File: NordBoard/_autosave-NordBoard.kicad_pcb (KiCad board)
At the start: 2 copper layers, 18 parts, among them SW1 SW_Push, SW10 SW_Push, SW11 SW_Push, SW12 SW_Push, SW13 SW_Push, SW14 SW_Push, SW17 SW_Push, SW18 SW_Push, SW19 SW_Push, SW20 SW_Push, SW21 SW_Push, SW3 SW_Push, SW4 SW_Push, SW5 SW_Push, SW6 SW_Push, SW7 SW_Push, SW8 SW_Push, U1 MOUDLE-SEEEDUINO-XIAO

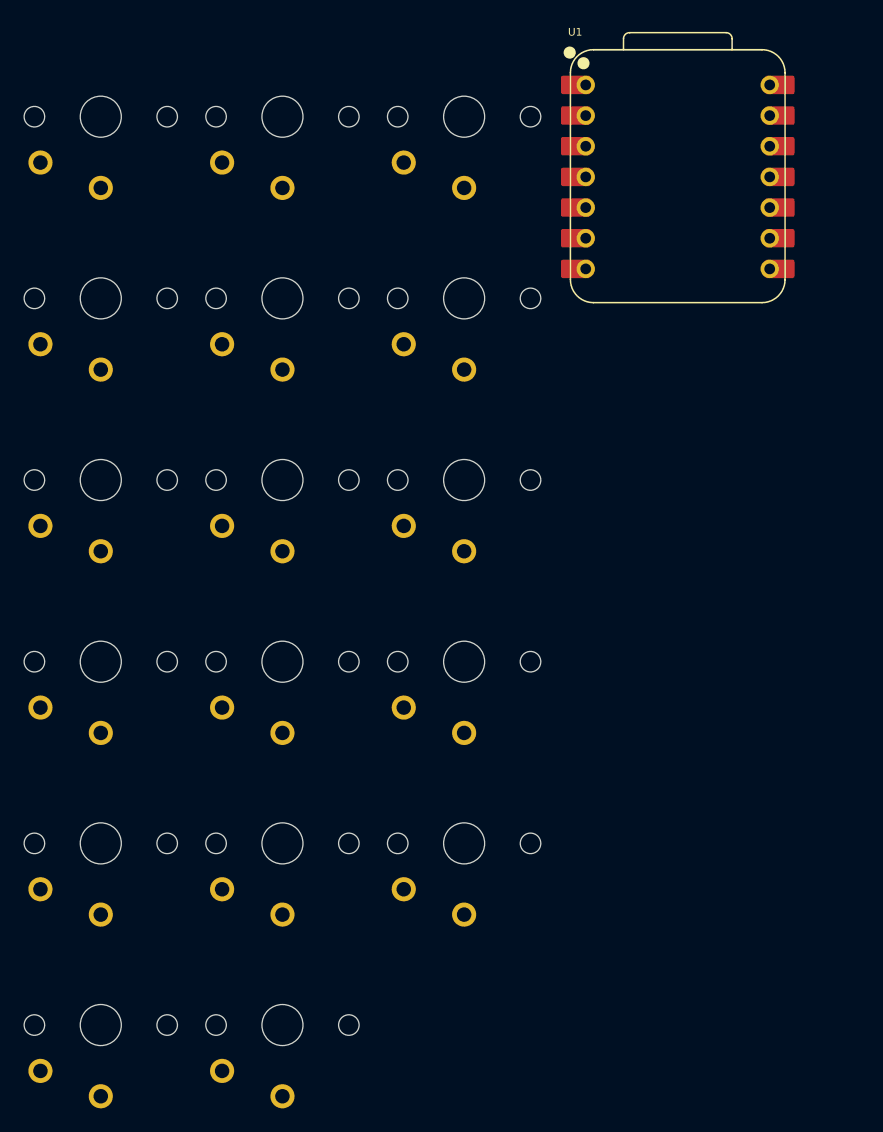
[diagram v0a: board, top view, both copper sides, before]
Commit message: feat: work on schem layout
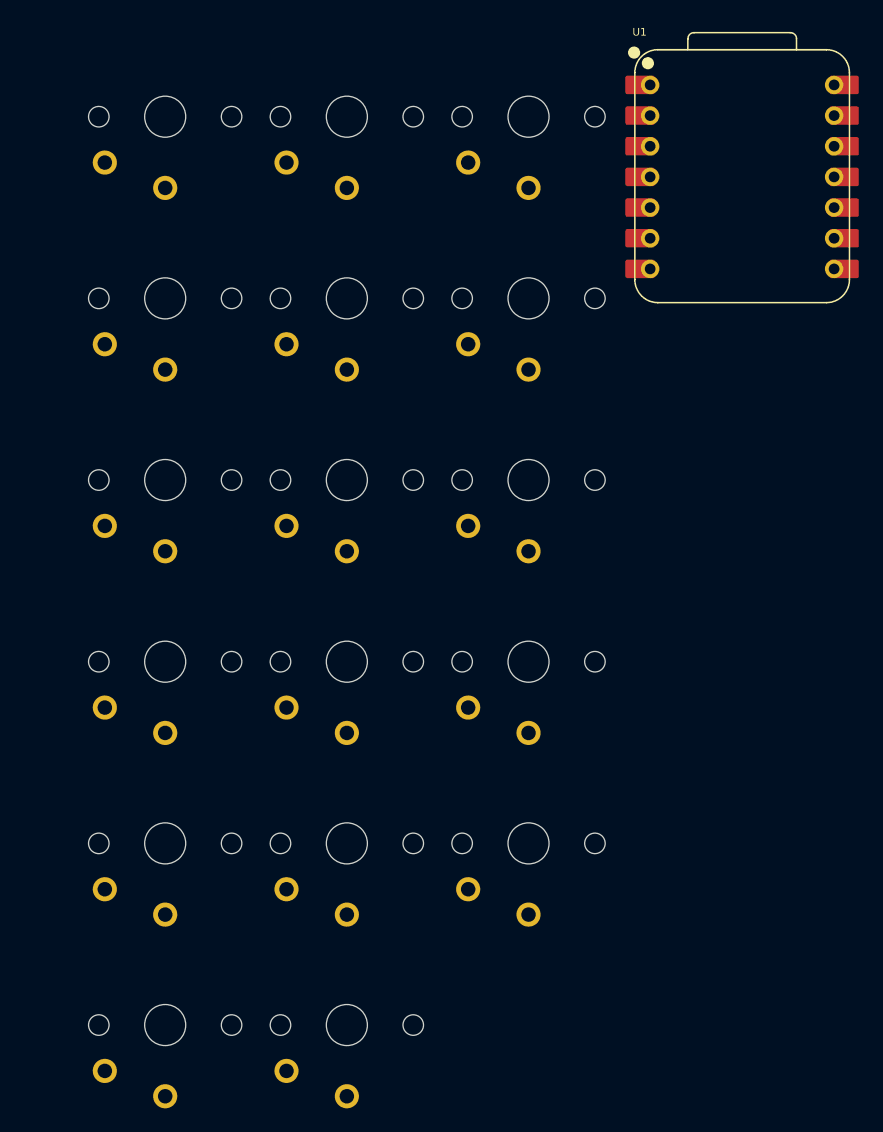
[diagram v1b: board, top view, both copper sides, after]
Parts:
- moved SW1 5.34 mm to (92.1, 43.9)
- moved SW3 5.34 mm to (92.1, 58.9)
- moved SW4 5.34 mm to (92.1, 74.0)
- moved SW5 5.34 mm to (92.1, 89.0)
- moved SW6 5.34 mm to (92.1, 104.1)
- moved SW7 5.34 mm to (92.1, 119.1)
- moved U1 5.34 mm to (139.9, 48.9)
- moved SW10 5.33 mm to (107.1, 58.9)
- moved SW11 5.33 mm to (107.1, 74.0)
- moved SW12 5.33 mm to (107.1, 89.0)
- moved SW13 5.33 mm to (107.1, 104.1)
- moved SW14 5.33 mm to (107.1, 119.1)
- moved SW17 5.33 mm to (122.2, 43.9)
- moved SW18 5.33 mm to (122.2, 58.9)
- moved SW19 5.33 mm to (122.2, 74.0)
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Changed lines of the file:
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@@
 	(footprint "PCM_marbastlib-choc:SW_choc_v1_1u"
 		(layer "F.Cu")
-		(at 86.749 73.9905)
+		(at 92.084 73.9905)
 		(descr "Footprint for Kailh Choc style switches")
 		(property "Reference" "SW4"
@@
 	(footprint "PCM_marbastlib-choc:SW_choc_v1_1u"
 		(layer "F.Cu")
-		(at 86.749 58.9405)
+		(at 92.084 58.9405)
 		(descr "Footprint for Kailh Choc style switches")
 		(property "Reference" "SW3"
@@
 	(footprint "PCM_marbastlib-choc:SW_choc_v1_1u"
 		(layer "F.Cu")
-		(at 116.849 43.8905)
+		(at 122.184 43.8905)
 		(descr "Footprint for Kailh Choc style switches")
 		(property "Reference" "SW17"
@@
 	(footprint "PCM_marbastlib-choc:SW_choc_v1_1u"
 		(layer "F.Cu")
-		(at 101.799 89.0405)
+		(at 107.134 89.0405)
 		(descr "Footprint for Kailh Choc style switches")
 		(property "Reference" "SW12"
@@
 	(footprint "PCM_marbastlib-choc:SW_choc_v1_1u"
 		(layer "F.Cu")
-		(at 116.849 89.0405)
+		(at 122.184 89.0405)
 		(descr "Footprint for Kailh Choc style switches")
 		(property "Reference" "SW20"
@@
 	(footprint "PCM_marbastlib-choc:SW_choc_v1_1u"
 		(layer "F.Cu")
-		(at 86.749 119.1405)
+		(at 92.084 119.1405)
 		(descr "Footprint for Kailh Choc style switches")
 		(property "Reference" "SW7"
@@
 	(footprint "PCM_marbastlib-choc:SW_choc_v1_1u"
 		(layer "F.Cu")
-		(at 116.849 73.9905)
+		(at 122.184 73.9905)
 		(descr "Footprint for Kailh Choc style switches")
 		(property "Reference" "SW19"
@@
 	(footprint "PCM_marbastlib-choc:SW_choc_v1_1u"
 		(layer "F.Cu")
-		(at 86.749 43.8905)
+		(at 92.084 43.8905)
 		(descr "Footprint for Kailh Choc style switches")
 		(property "Reference" "SW1"
@@
 	(footprint "PCM_marbastlib-choc:SW_choc_v1_1u"
 		(layer "F.Cu")
-		(at 101.799 43.8905)
+		(at 107.134 43.8905)
 		(descr "Footprint for Kailh Choc style switches")
 		(property "Reference" "SW8"
@@
 	(footprint "PCM_marbastlib-choc:SW_choc_v1_1u"
 		(layer "F.Cu")
-		(at 116.849 104.0905)
+		(at 122.184 104.0905)
 		(descr "Footprint for Kailh Choc style switches")
 		(property "Reference" "SW21"
@@
 	(footprint "PCM_marbastlib-choc:SW_choc_v1_1u"
 		(layer "F.Cu")
-		(at 86.749 89.0405)
+		(at 92.084 89.0405)
 		(descr "Footprint for Kailh Choc style switches")
 		(property "Reference" "SW5"
@@
 	(footprint "PCM_marbastlib-choc:SW_choc_v1_1u"
 		(layer "F.Cu")
-		(at 101.799 119.1405)
+		(at 107.134 119.1405)
 		(descr "Footprint for Kailh Choc style switches")
 		(property "Reference" "SW14"
@@
 	(footprint "PCM_marbastlib-choc:SW_choc_v1_1u"
 		(layer "F.Cu")
-		(at 101.799 104.0905)
+		(at 107.134 104.0905)
 		(descr "Footprint for Kailh Choc style switches")
 		(property "Reference" "SW13"
@@
 	(footprint "Seeed Studio XIAO Series Library:XIAO-RP2040-DIP"
 		(layer "F.Cu")
-		(at 134.545 48.88)
+		(at 139.88 48.88)
 		(property "Reference" "U1"
 			(at -8.5 -12 0)
@@
 	(footprint "PCM_marbastlib-choc:SW_choc_v1_1u"
 		(layer "F.Cu")
-		(at 101.799 58.9405)
+		(at 107.134 58.9405)
 		(descr "Footprint for Kailh Choc style switches")
 		(property "Reference" "SW10"
@@
 	(footprint "PCM_marbastlib-choc:SW_choc_v1_1u"
 		(layer "F.Cu")
-		(at 101.799 73.9905)
+		(at 107.134 73.9905)
 		(descr "Footprint for Kailh Choc style switches")
 		(property "Reference" "SW11"
@@
 	(footprint "PCM_marbastlib-choc:SW_choc_v1_1u"
 		(layer "F.Cu")
-		(at 116.849 58.9405)
+		(at 122.184 58.9405)
 		(descr "Footprint for Kailh Choc style switches")
 		(property "Reference" "SW18"
@@
 	(footprint "PCM_marbastlib-choc:SW_choc_v1_1u"
 		(layer "F.Cu")
-		(at 86.749 104.0905)
+		(at 92.084 104.0905)
 		(descr "Footprint for Kailh Choc style switches")
 		(property "Reference" "SW6"
